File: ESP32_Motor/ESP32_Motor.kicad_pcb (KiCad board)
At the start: 2 copper layers, 80.5 x 63.2 mm, 18 parts, among them J1 Screw_Terminal_01x02, J2 Screw_Terminal_01x02, Q1 IRLML9301, Q2 BC847, U2 YD-ESP32-S3

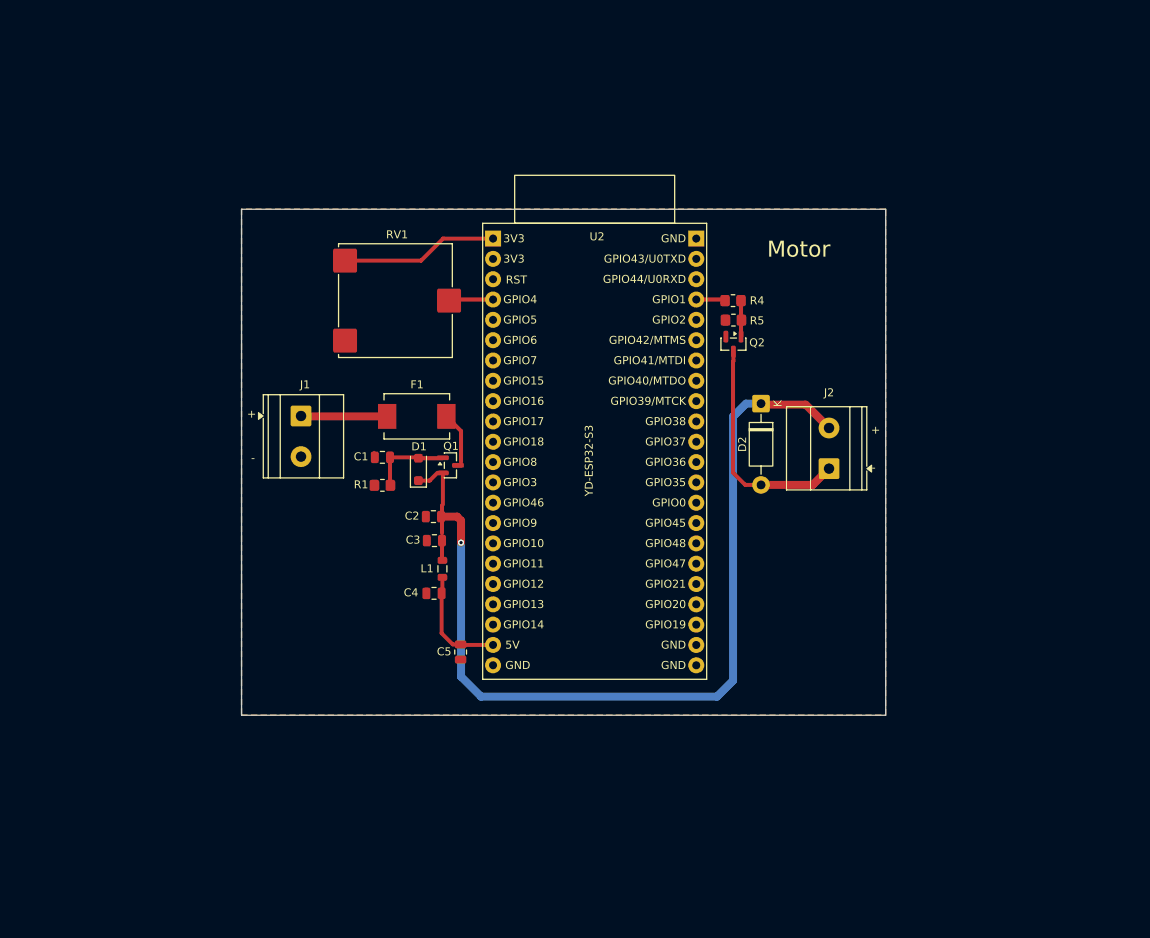
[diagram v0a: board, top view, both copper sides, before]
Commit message: M_5_5_26_08_26
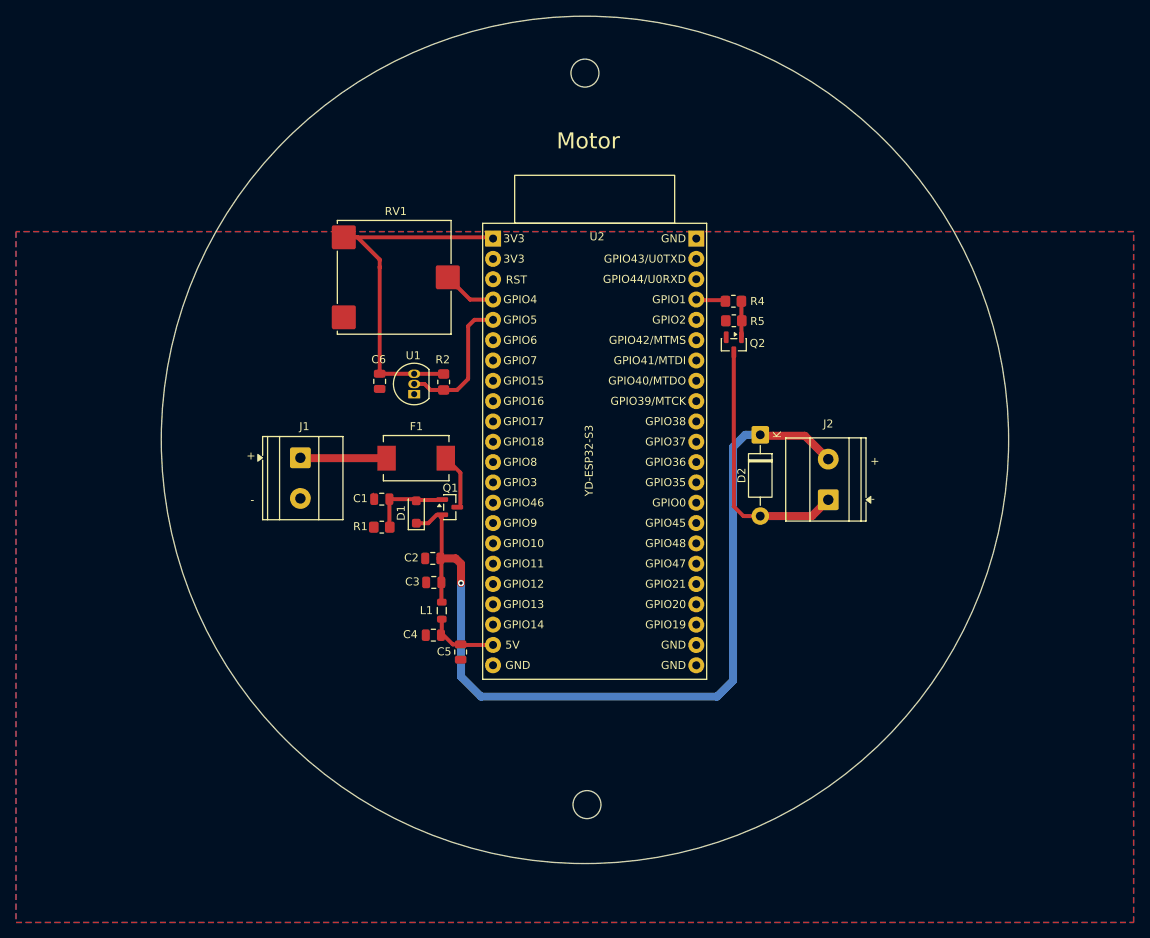
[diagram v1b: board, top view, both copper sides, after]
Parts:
- added C6: 0.1u, Capacitor_SMD:C_0805_2012Metric, F.Cu at (116.6, 89.8)
- added R2: 4.7K, Resistor_SMD:R_0805_2012Metric_Pad1.20x1.40mm_HandSolder, F.Cu at (124.6, 89.9)
- added REF**: MountingHole_3.5mm, MountingHole:MountingHole_3.5mm, F.Cu at (142.5, 142.7)
- added REF**: MountingHole_3.5mm, MountingHole:MountingHole_3.5mm, F.Cu at (142.2, 51.3)
- added U1: DS18B20, Package_TO_SOT_THT:TO-92_Inline, F.Cu at (120.9, 91.4)
- D1: value BZT52B12V -> BZT52B5V6
- moved D1 5.33 mm to (121.2, 106.2)
- moved C1 5.23 mm to (116.8, 104.6)
- moved C2 5.23 mm to (123.2, 112.0)
- moved C3 5.23 mm to (123.3, 115.0)
- moved C4 5.23 mm to (123.3, 121.6)
- moved F1 5.23 mm to (121.1, 99.4)
- moved J1 5.23 mm to (106.7, 99.4)
- moved L1 5.23 mm to (124.3, 118.5)
- moved Q1 5.23 mm to (125.3, 105.6)
- moved R1 5.23 mm to (116.8, 108.1)
- moved D2 3.90 mm to (164.2, 96.5)
- moved J2 3.90 mm to (172.7, 104.6)
- moved RV1 2.92 mm to (118.6, 76.8)
- moved Q2 0.09 mm to (160.8, 85.3)
- moved R4 0.09 mm to (160.8, 79.8)
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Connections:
- net Net-(RV1-Pad3) renamed +3V3
- U2 pad 5: unconnected-(U2-GPIO5-Pad5) -> Net-(U1-DQ)
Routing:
- net +3V3: track 19.6 -> 45.0 mm
- net Net-(U1-DQ): track 0.00 -> 17.7 mm
- net +5VP: track 118.6 -> 111.1 mm
- net +5V: track 14.1 -> 9.08 mm
- net Net-(D2-A): track 29.1 -> 32.9 mm
- net Net-(U2-GPIO4): track 5.56 -> 7.50 mm
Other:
- board size 80.5 x 63.2 mm -> 105.9 x 105.9 mm
